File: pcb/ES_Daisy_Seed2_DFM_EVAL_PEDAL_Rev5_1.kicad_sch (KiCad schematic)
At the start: 32 parts, among them Q1 3904, Q5 3904, U11 H11L1, U14 USBLC6-2SC6, U4 GT-USB-7010ASV, U5 G6K-2F-Y-TR DC3, U6 G6K-2F-Y-TR DC3

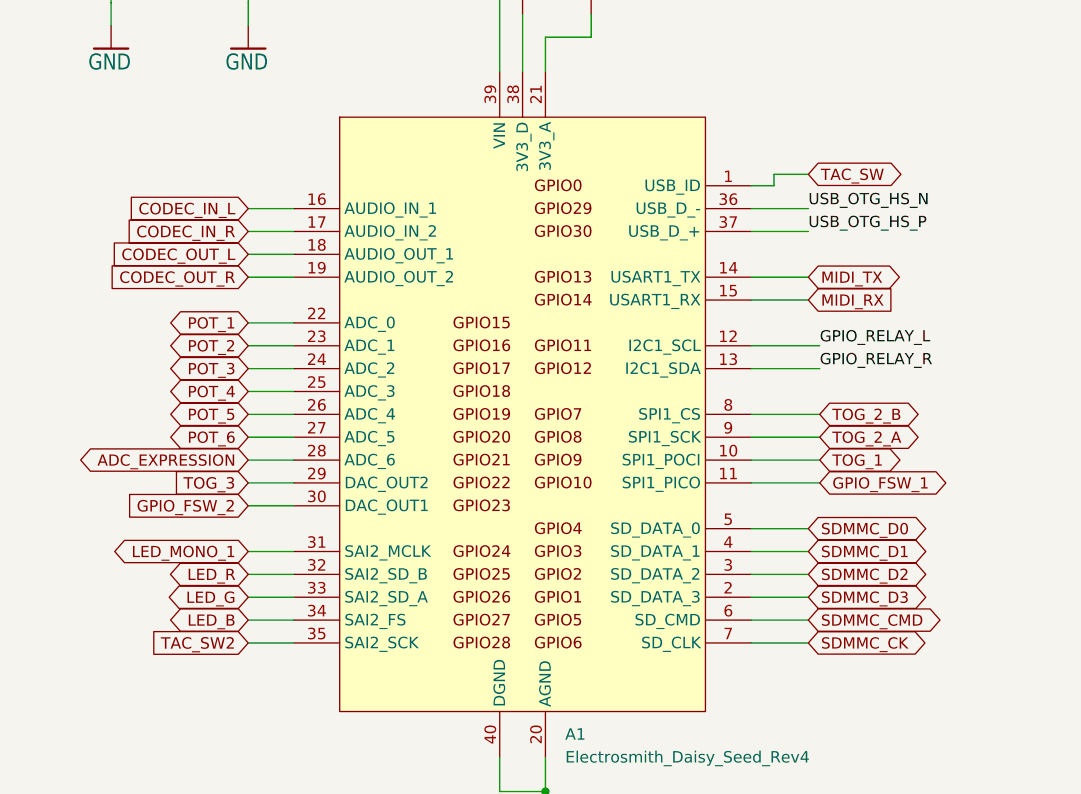
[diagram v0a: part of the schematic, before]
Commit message: fully routed.
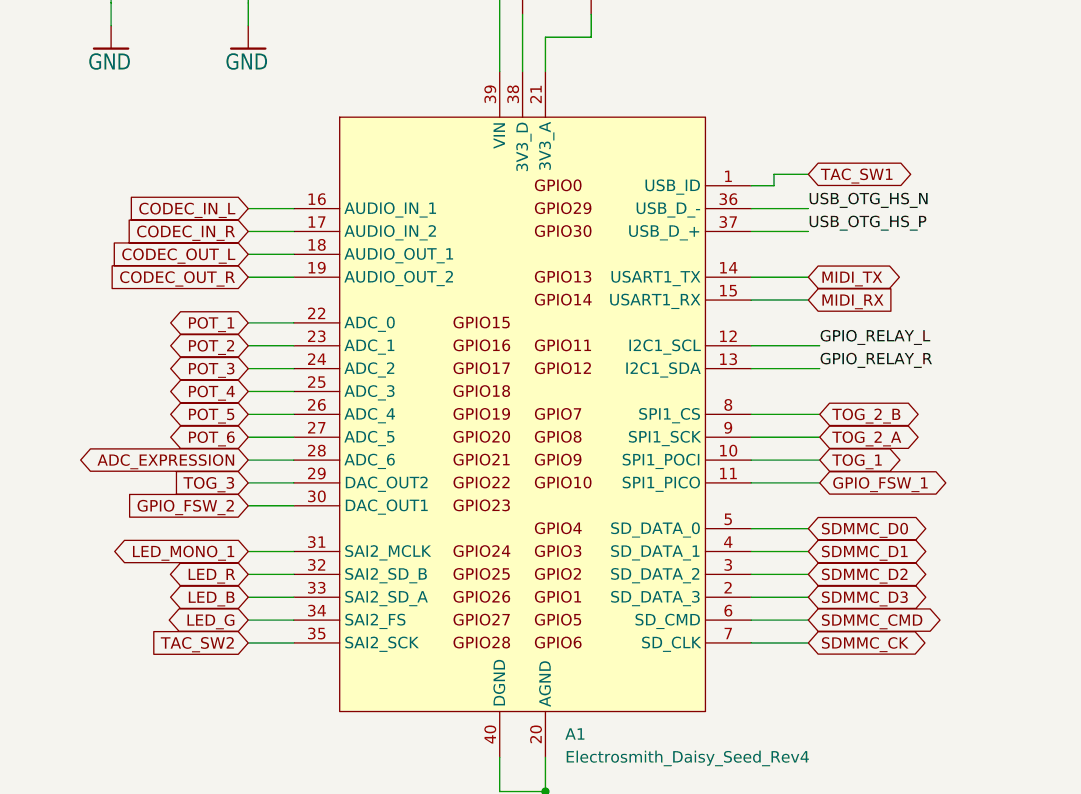
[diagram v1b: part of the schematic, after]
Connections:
- net LED_B: now also A1.33 (SAI2_SD_A); no longer A1.34 (SAI2_FS)
- net LED_G: now also A1.34 (SAI2_FS); no longer A1.33 (SAI2_SD_A)
- net TAC_SW renamed TAC_SW1
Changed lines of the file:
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@@
 		)
 	)
-	(global_label "TAC_SW"
+	(global_label "TAC_SW1"
 		(shape bidirectional)
 		(at 138.43 78.74 0)
@@
 		)
 		(property "Intersheetrefs" "${INTERSHEET_REFS}"
-			(at 149.2599 78.74 0)
+			(at 150.4452 78.74 0)
 			(effects
 				(font
@@
 	(global_label "LED_G"
 		(shape bidirectional)
+		(at 76.2 128.27 180)
+		(fields_autoplaced yes)
+		(effects
+			(font
+				(size 1.2446 1.2446)
+			)
+			(justify right)
+		)
+		(property "Intersheetrefs" "${INTERSHEET_REFS}"
+			(at 66.6147 128.27 0)
+			(effects
+				(font
+					(size 1.27 1.27)
+				)
+				(justify right)
+				(hide yes)
+			)
+		)
+	)
+	(global_label "AUDIO_DSP_LEFT"
+		(shape bidirectional)
+		(at 288.29 209.55 0)
+		(fields_autoplaced yes)
+		(effects
+			(font
+				(size 1.2446 1.2446)
+			)
+			(justify left)
+		)
+		(property "Intersheetrefs" "${INTERSHEET_REFS}"
+			(at 307.5359 209.55 0)
+			(effects
+				(font
+					(size 1.27 1.27)
+				)
+				(justify left)
+				(hide yes)
+			)
+		)
+	)
+	(global_label "POT_6"
+		(shape bidirectional)
+		(at 76.2 107.95 180)
+		(fields_autoplaced yes)
+		(effects
+			(font
+				(size 1.2446 1.2446)
+			)
+			(justify right)
+		)
+		(property "Intersheetrefs" "${INTERSHEET_REFS}"
+			(at 66.5554 107.95 0)
+			(effects
+				(font
+					(size 1.27 1.27)
+				)
+				(justify right)
+				(hide yes)
+			)
+		)
+	)
+	(global_label "+9V"
+		(shape bidirectional)
+		(at 43.18 46.99 180)
+		(fields_autoplaced yes)
+		(effects
+			(font
+				(size 1.2446 1.2446)
+			)
+			(justify right)
+		)
+		(property "Intersheetrefs" "${INTERSHEET_REFS}"
+			(at 35.3728 46.99 0)
+			(effects
+				(font
+					(size 1.27 1.27)
+				)
+				(justify right)
+				(hide yes)
+			)
+		)
+	)
+	(global_label "TOG_2_A"
+		(shape bidirectional)
+		(at 139.7 107.95 0)
+		(fields_autoplaced yes)
+		(effects
+			(font
+				(size 1.2446 1.2446)
+			)
+			(justify left)
+		)
+		(property "Intersheetrefs" "${INTERSHEET_REFS}"
+			(at 151.3597 107.95 0)
+			(effects
+				(font
+					(size 1.27 1.27)
+				)
+				(justify left)
+				(hide yes)
+			)
+		)
+	)
+	(global_label "SDMMC_D0"
+		(shape bidirectional)
+		(at 138.43 118.11 0)
+		(fields_autoplaced yes)
+		(effects
+			(font
+				(size 1.2446 1.2446)
+			)
+			(justify left)
+		)
+		(property "Intersheetrefs" "${INTERSHEET_REFS}"
+			(at 152.3417 118.11 0)
+			(effects
+				(font
+					(size 1.27 1.27)
+				)
+				(justify left)
+				(hide yes)
+			)
+		)
+	)
+	(global_label "AUDIO_IN_RIGHT"
+		(shape bidirectional)
+		(at 384.81 207.01 0)
+		(fields_autoplaced yes)
+		(effects
+			(font
+				(size 1.2446 1.2446)
+			)
+			(justify left)
+		)
+		(property "Intersheetrefs" "${INTERSHEET_REFS}"
+			(at 403.4634 207.01 0)
+			(effects
+				(font
+					(size 1.27 1.27)
+				)
+				(justify left)
+				(hide yes)
+			)
+		)
+	)
+	(global_label "LED_B"
+		(shape bidirectional)
 		(at 76.2 125.73 180)
 		(fields_autoplaced yes)
@@
 			(effects
 				(font
-					(size 1.27 1.27)
-				)
-				(justify right)
-				(hide yes)
-			)
-		)
-	)
-	(global_label "AUDIO_DSP_LEFT"
-		(shape bidirectional)
-		(at 288.29 209.55 0)
-		(fields_autoplaced yes)
-		(effects
-			(font
-				(size 1.2446 1.2446)
-			)
-			(justify left)
-		)
-		(property "Intersheetrefs" "${INTERSHEET_REFS}"
-			(at 307.5359 209.55 0)
-			(effects
-				(font
-					(size 1.27 1.27)
-				)
-				(justify left)
-				(hide yes)
-			)
-		)
-	)
-	(global_label "POT_6"
-		(shape bidirectional)
-		(at 76.2 107.95 180)
-		(fields_autoplaced yes)
-		(effects
-			(font
-				(size 1.2446 1.2446)
-			)
-			(justify right)
-		)
-		(property "Intersheetrefs" "${INTERSHEET_REFS}"
-			(at 66.5554 107.95 0)
-			(effects
-				(font
-					(size 1.27 1.27)
-				)
-				(justify right)
-				(hide yes)
-			)
-		)
-	)
-	(global_label "+9V"
-		(shape bidirectional)
-		(at 43.18 46.99 180)
-		(fields_autoplaced yes)
-		(effects
-			(font
-				(size 1.2446 1.2446)
-			)
-			(justify right)
-		)
-		(property "Intersheetrefs" "${INTERSHEET_REFS}"
-			(at 35.3728 46.99 0)
-			(effects
-				(font
-					(size 1.27 1.27)
-				)
-				(justify right)
-				(hide yes)
-			)
-		)
-	)
-	(global_label "TOG_2_A"
-		(shape bidirectional)
-		(at 139.7 107.95 0)
-		(fields_autoplaced yes)
-		(effects
-			(font
-				(size 1.2446 1.2446)
-			)
-			(justify left)
-		)
-		(property "Intersheetrefs" "${INTERSHEET_REFS}"
-			(at 151.3597 107.95 0)
-			(effects
-				(font
-					(size 1.27 1.27)
-				)
-				(justify left)
-				(hide yes)
-			)
-		)
-	)
-	(global_label "SDMMC_D0"
-		(shape bidirectional)
-		(at 138.43 118.11 0)
-		(fields_autoplaced yes)
-		(effects
-			(font
-				(size 1.2446 1.2446)
-			)
-			(justify left)
-		)
-		(property "Intersheetrefs" "${INTERSHEET_REFS}"
-			(at 152.3417 118.11 0)
-			(effects
-				(font
-					(size 1.27 1.27)
-				)
-				(justify left)
-				(hide yes)
-			)
-		)
-	)
-	(global_label "AUDIO_IN_RIGHT"
-		(shape bidirectional)
-		(at 384.81 207.01 0)
-		(fields_autoplaced yes)
-		(effects
-			(font
-				(size 1.2446 1.2446)
-			)
-			(justify left)
-		)
-		(property "Intersheetrefs" "${INTERSHEET_REFS}"
-			(at 403.4634 207.01 0)
-			(effects
-				(font
-					(size 1.27 1.27)
-				)
-				(justify left)
-				(hide yes)
-			)
-		)
-	)
-	(global_label "LED_B"
-		(shape bidirectional)
-		(at 76.2 128.27 180)
-		(fields_autoplaced yes)
-		(effects
-			(font
-				(size 1.2446 1.2446)
-			)
-			(justify right)
-		)
-		(property "Intersheetrefs" "${INTERSHEET_REFS}"
-			(at 66.6147 128.27 0)
-			(effects
-				(font
